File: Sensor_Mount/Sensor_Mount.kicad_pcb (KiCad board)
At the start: 2 copper layers, 150 x 56 mm, 5 parts, among them J1 Screw_Terminal_01x10

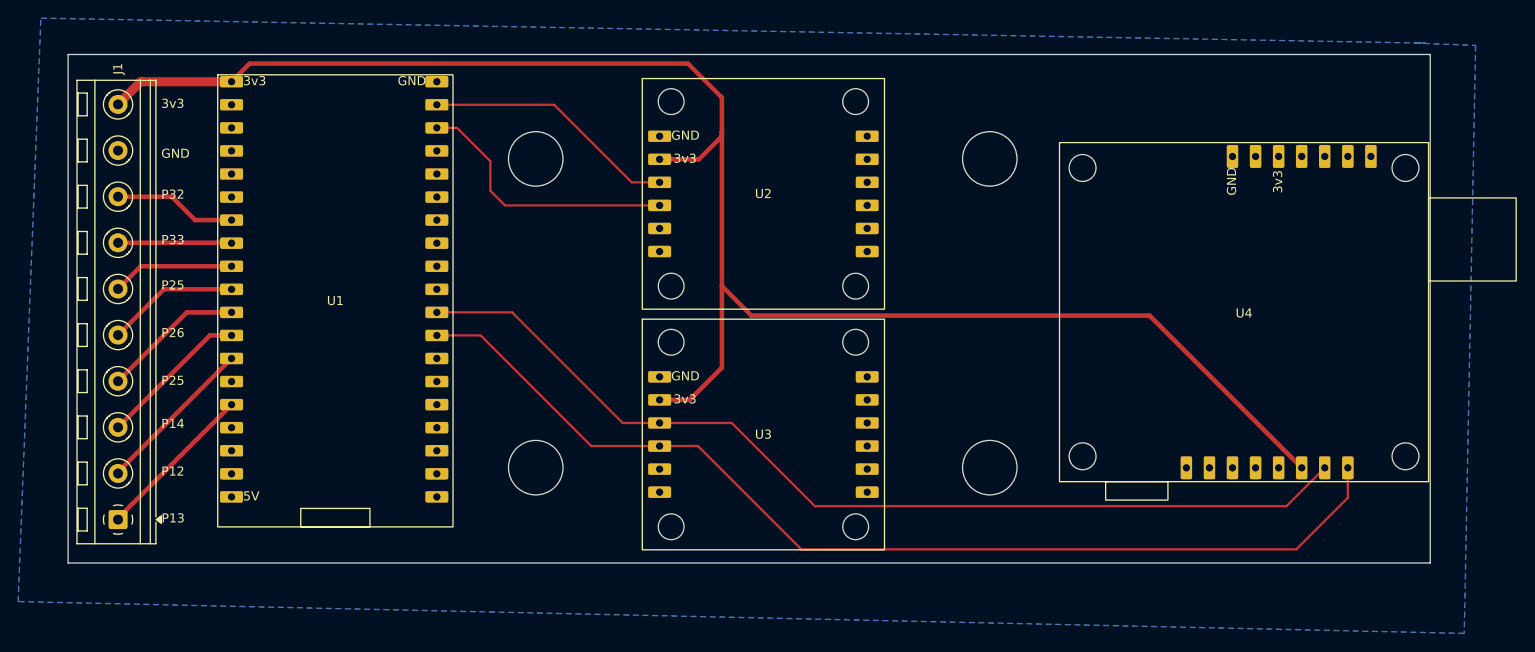
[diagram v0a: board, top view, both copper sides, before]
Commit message: Ordered Parts
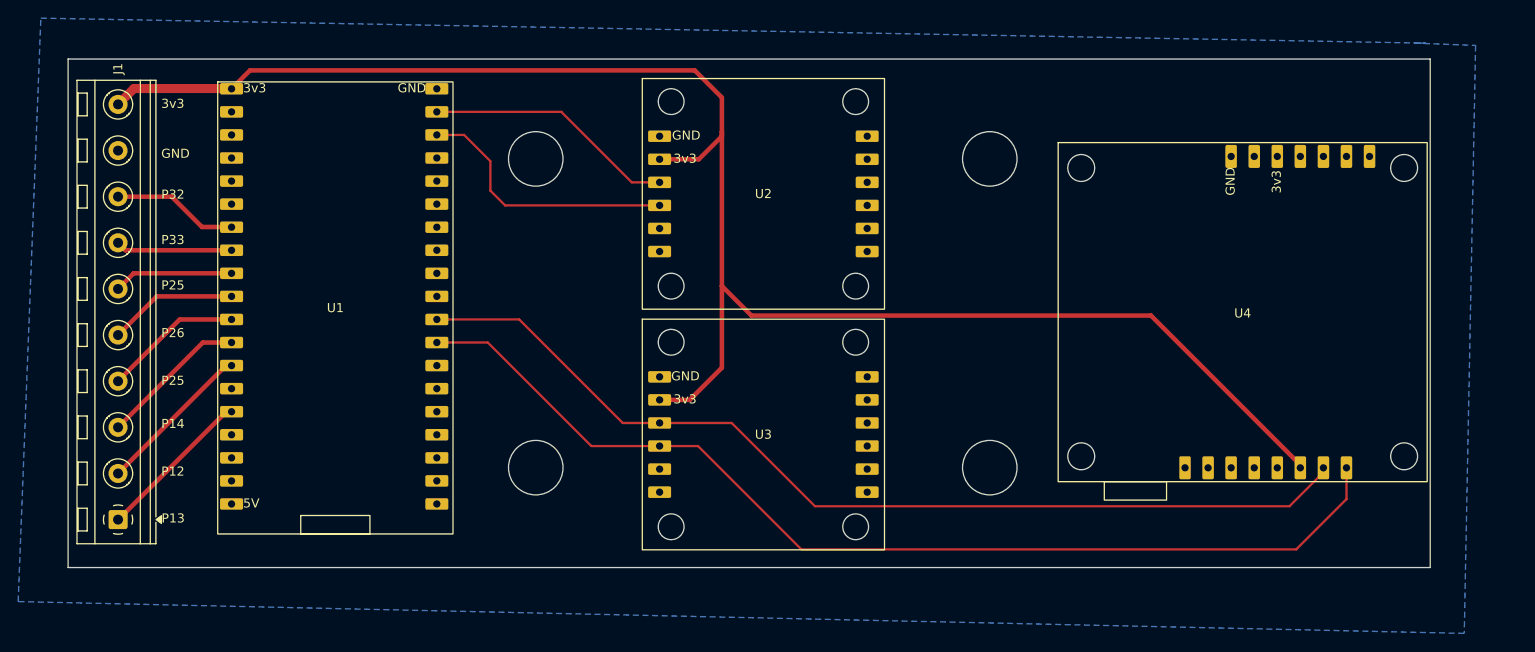
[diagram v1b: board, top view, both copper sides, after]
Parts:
- moved U1 0.78 mm to (112.4, 63.4)
- moved U4 0.15 mm to (212.3, 64.0)
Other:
- outline, holes or cut-outs redrawn
